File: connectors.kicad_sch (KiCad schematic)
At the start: 4 parts, among them J1 Conn_01x04_Pin, J2 Conn_01x04_Pin, J3 Conn_01x09_Pin, J4 Conn_02x03_Odd_Even

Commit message: associated symbol & footprint
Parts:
- J1, J2: footprint (none) -> Connector_PinHeader_2.54mm:PinHeader_1x04_P2.54mm_Vertical
- J3: footprint (none) -> Connector_PinHeader_2.54mm:PinHeader_1x09_P2.54mm_Vertical
- J4: footprint (none) -> Connector_PinHeader_2.54mm:PinHeader_2x03_P2.54mm_Vertical
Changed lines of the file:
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@@
 			)
 		)
-		(property "Footprint" ""
+		(property "Footprint" "Connector_PinHeader_2.54mm:PinHeader_1x04_P2.54mm_Vertical"
 			(at 113.03 67.31 0)
 			(effects
@@
 			)
 		)
-		(property "Footprint" ""
+		(property "Footprint" "Connector_PinHeader_2.54mm:PinHeader_1x09_P2.54mm_Vertical"
 			(at 69.85 69.85 0)
 			(effects
@@
 			)
 		)
-		(property "Footprint" ""
+		(property "Footprint" "Connector_PinHeader_2.54mm:PinHeader_2x03_P2.54mm_Vertical"
 			(at 142.24 71.12 0)
 			(effects
@@
 			)
 		)
-		(property "Footprint" ""
+		(property "Footprint" "Connector_PinHeader_2.54mm:PinHeader_1x04_P2.54mm_Vertical"
 			(at 92.71 68.58 0)
 			(effects

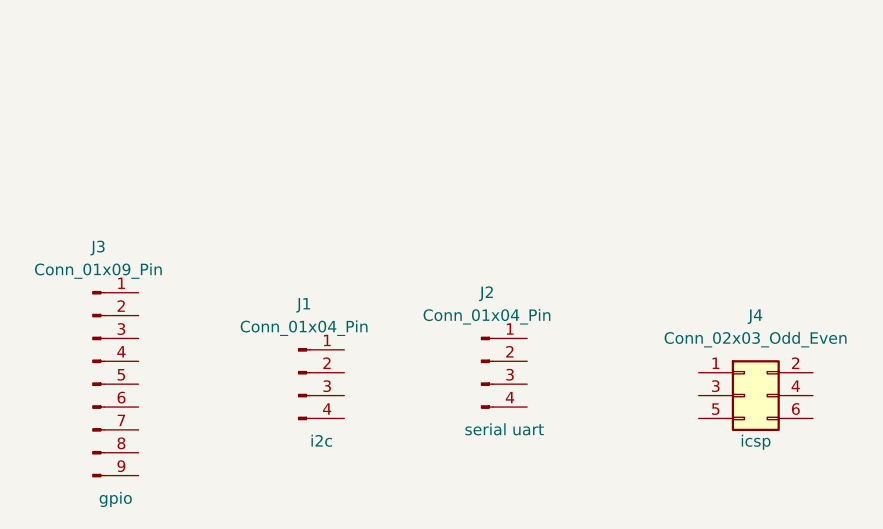
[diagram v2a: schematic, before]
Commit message: completed wiring
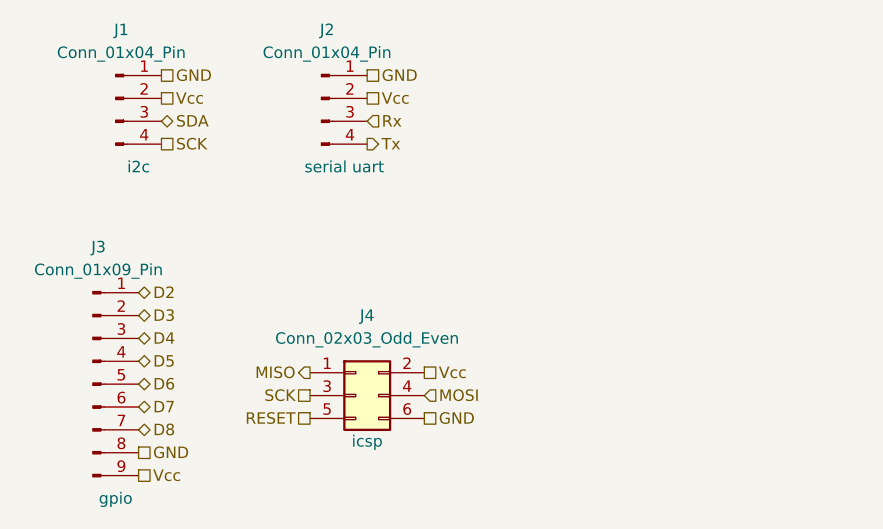
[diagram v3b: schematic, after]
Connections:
- net GND: now reaches J2.1 (Pin_1)
- net GND: now also J1.1 (Pin_1), J3.8 (Pin_8), J4.6 (Pin_6)
- net Vcc: now reaches J2.2 (Pin_2)
- net Vcc: now also J1.2 (Pin_2), J3.9 (Pin_9), J4.2 (Pin_2)
- net Rx: now reaches J2.3 (Pin_3)
- net Tx: now reaches J2.4 (Pin_4)
- net D2: now reaches J3.1 (Pin_1)
- net D3: now reaches J3.2 (Pin_2)
- net D4: now reaches J3.3 (Pin_3)
- net D5: now reaches J3.4 (Pin_4)
- net D6: now reaches J3.5 (Pin_5)
- net D7: now reaches J3.6 (Pin_6)
- net D8: now reaches J3.7 (Pin_7)
- net MISO: now reaches J4.1 (Pin_1)
- net SCK: now reaches J4.3 (Pin_3)
- net SCK: now also J1.4 (Pin_4)
- net MOSI: now reaches J4.4 (Pin_4)
- net RESET: now reaches J4.5 (Pin_5)
- net SDA: now reaches J1.3 (Pin_3)
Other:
- moved on the sheet: J1, J2, J4
